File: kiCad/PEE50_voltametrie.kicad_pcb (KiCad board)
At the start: 2 copper layers, 75.3 x 66.3 mm, 48 parts, among them IC2 TPS7A2045PDBVR, IC3 TMUX1109PWR, IC5 ADS1113IDGSR, IC6 DAC80501MDGSR, IC7 LMP7702MA_NOPB, IC8 DS18B20+, J1 2201778-1, J2 USB_B_Micro, J4 Conn_02x03_Odd_Even, U1 ESP32-DEVKITC-32D

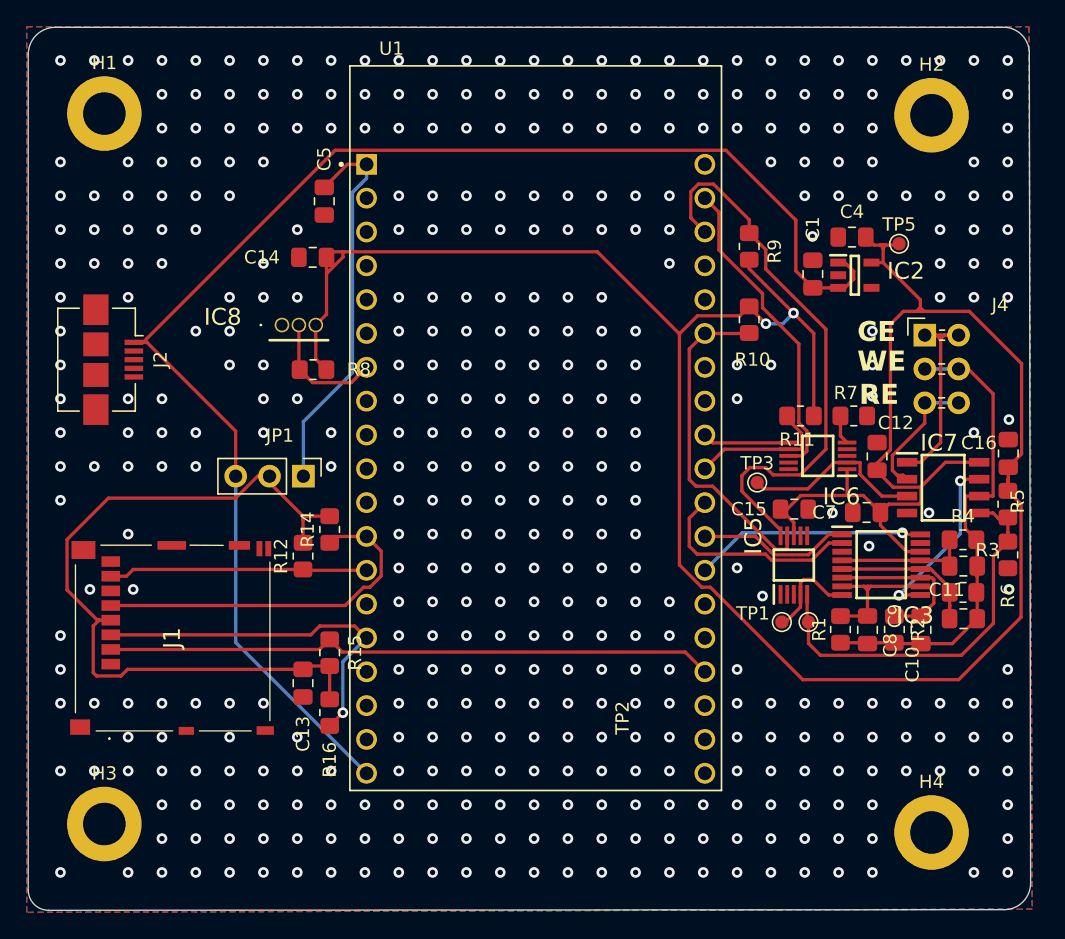
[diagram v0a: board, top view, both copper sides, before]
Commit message: final pcb update
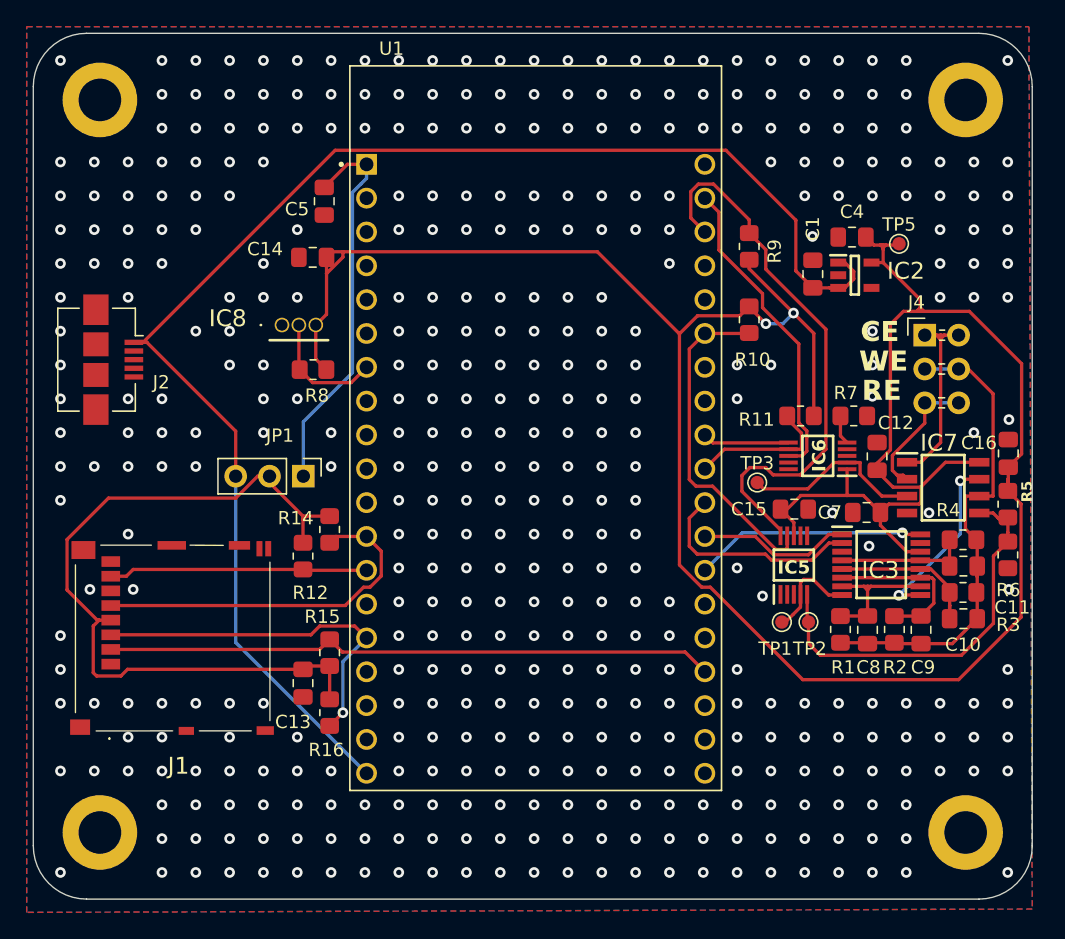
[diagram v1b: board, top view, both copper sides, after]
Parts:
- moved H2 2.81 mm to (205.0, 72.0)
- moved H4 2.56 mm to (205.0, 127.0)
- moved H1 1.08 mm to (140.0, 72.0)
- moved H3 0.72 mm to (140.0, 127.0)
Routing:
- net GND: vias 434 -> 432
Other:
- board size 75.3 x 66.3 mm -> 75 x 65 mm
- board text added: "PEE50 Juni 2023 Voltammetrie"
- board text removed: "PEE50 Mei 2023 Voltametrie"
